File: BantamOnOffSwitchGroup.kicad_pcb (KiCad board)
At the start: 2 copper layers, 14.6 x 34 mm, 4 parts, among them J1 Conn_01x02_Male, J2 Conn_01x04_Male, SW1 SW_Push_DPDT

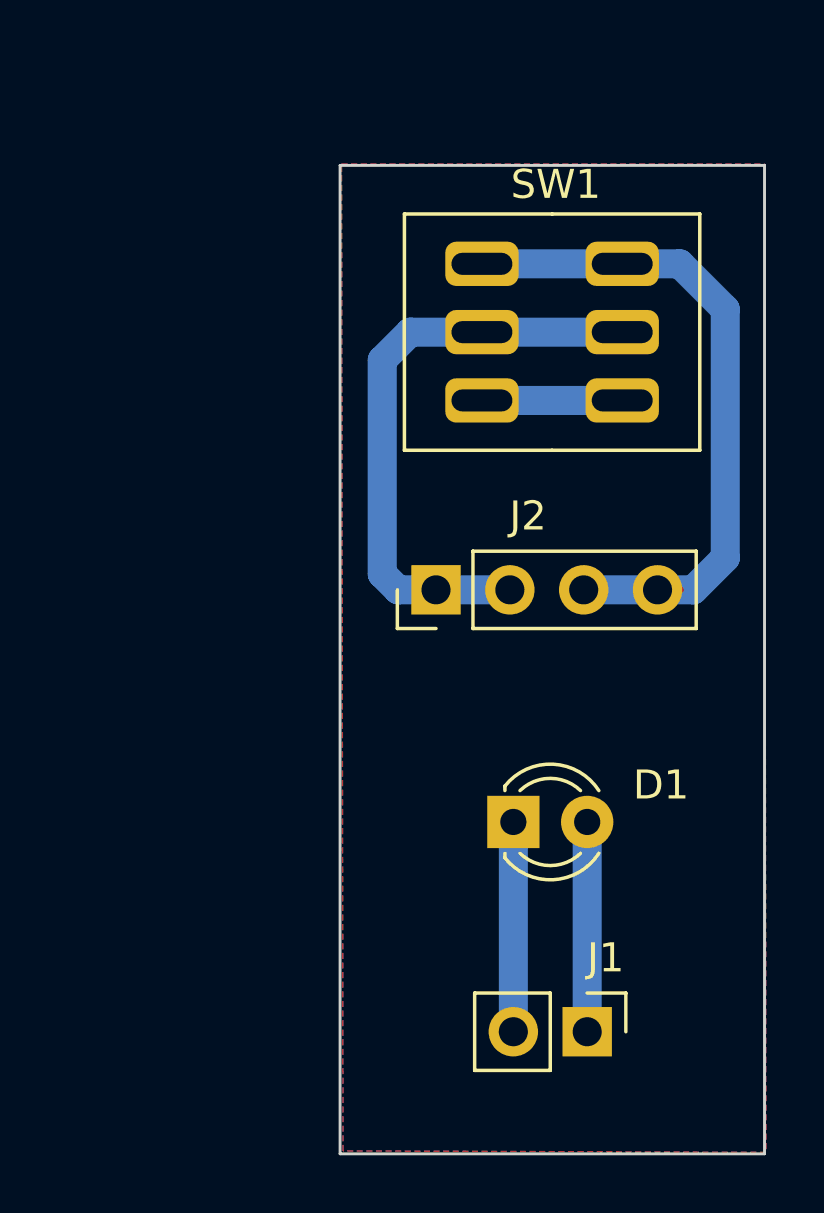
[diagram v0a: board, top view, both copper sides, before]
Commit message: gbr and drill files created
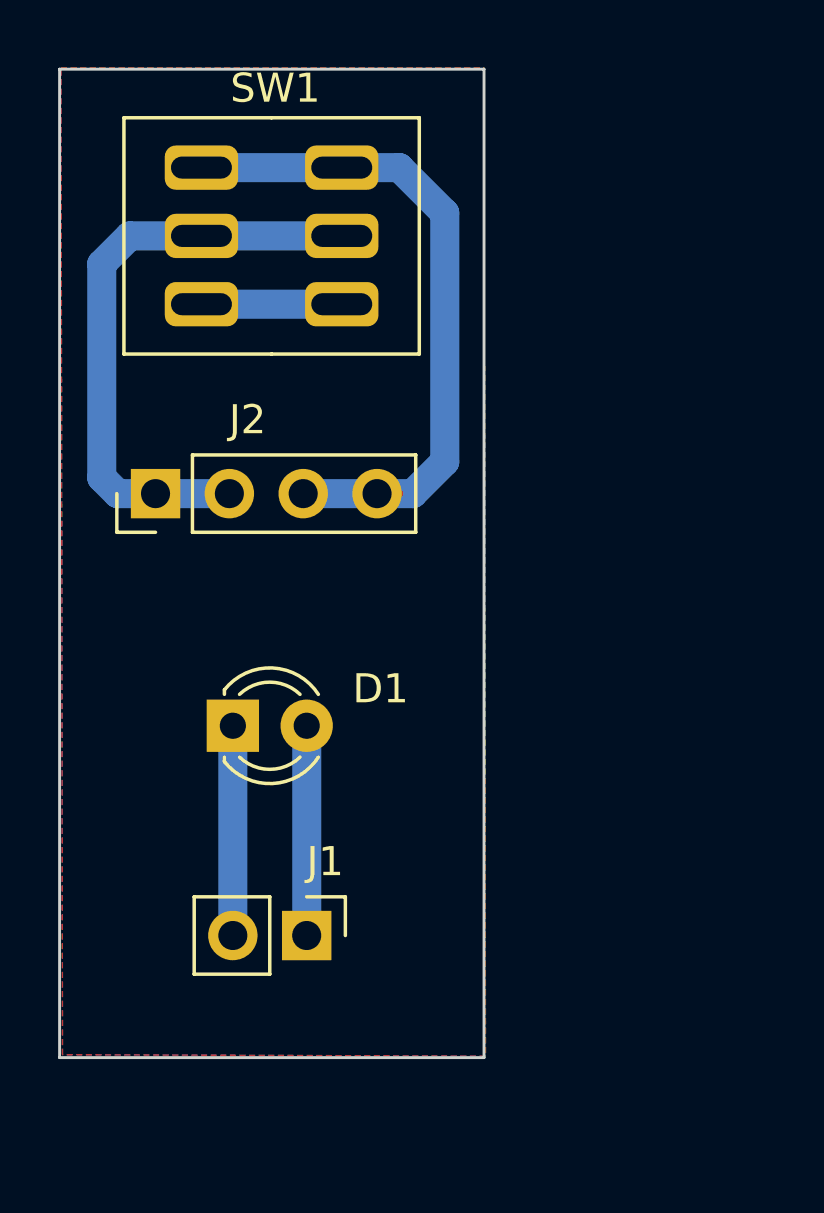
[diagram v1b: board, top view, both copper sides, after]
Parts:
- moved D1 10.2 mm to (136.2, 103.1)
- moved J1 10.2 mm to (138.8, 110.3)
- moved SW1 10.2 mm to (137.5, 86.2)
- moved J2 10.2 mm to (133.6, 95.1)
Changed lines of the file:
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@@
 		(legacy_teardrops no)
 	)
-	(paper "A4")
+	(paper "A")
+	(title_block
+		(title "Bantamp Power Switch Group")
+		(date "2024-03-06")
+		(company "RoboWidgets")
+	)
 	(layers
 		(0 "F.Cu" signal)
@@
 			(outputformat 1)
 			(mirror no)
-			(drillshape 1)
+			(drillshape 0)
 			(scaleselection 1)
-			(outputdirectory "")
+			(outputdirectory "ouput/")
 		)
 	)
@@
 	(footprint "Connector_PinHeader_2.54mm:PinHeader_1x04_P2.54mm_Vertical"
 		(layer "F.Cu")
-		(at 143.2 98.4 90)
+		(at 133.551824 95.090218 90)
 		(descr "Through hole straight pin header, 1x04, 2.54mm pitch, single row")
 		(tags "Through hole pin header THT 1x04 2.54mm single row")
@@
 	(footprint "LED_THT:LED_D3.0mm"
 		(layer "F.Cu")
-		(at 145.86 106.3845)
+		(at 136.211824 103.074718)
 		(descr "LED, diameter 3.0mm, 2 pins")
 		(tags "LED diameter 3.0mm 2 pins")
@@
 	(footprint "Connector_PinHeader_2.54mm:PinHeader_1x02_P2.54mm_Vertical"
 		(layer "F.Cu")
-		(at 148.4 113.6 -90)
+		(at 138.751824 110.290218 -90)
 		(descr "Through hole straight pin header, 1x02, 2.54mm pitch, single row")
 		(tags "Through hole pin header THT 1x02 2.54mm single row")
@@
 	(footprint "Kidwidgets:Toggle_DPDT"
 		(layer "F.Cu")
-		(at 147.193 89.535)
+		(at 137.544824 86.225218)
 		(property "Reference" "SW1"
 			(at 0.127 -5.08 0)
@@
 	)
 	(gr_rect
-		(start 139.9 83.8)
-		(end 154.5 117.8)
+		(start 130.251824 80.490218)
+		(end 144.851824 114.490218)
 		(stroke
 			(width 0.1)
@@
 	)
 	(segment
-		(start 145.86 106.3845)
-		(end 145.86 113.6)
+		(start 136.211824 103.074718)
+		(end 136.211824 110.290218)
 		(width 1)
 		(layer "B.Cu")
@@
 	)
 	(segment
-		(start 148.4 106.3845)
-		(end 148.4 113.6)
+		(start 138.751824 103.074718)
+		(end 138.751824 110.290218)
 		(width 1)
 		(layer "B.Cu")
@@
 	)
 	(segment
-		(start 143.2 98.4)
-		(end 145.74 98.4)
+		(start 133.551824 95.090218)
+		(end 136.091824 95.090218)
 		(width 1)
 		(layer "B.Cu")
@@
 	)
 	(segment
-		(start 144.78 89.535)
-		(end 142.315 89.535)
+		(start 135.131824 86.225218)
+		(end 132.666824 86.225218)
 		(width 1)
 		(layer "B.Cu")
@@
 	)
 	(segment
-		(start 141.35 97.85)
-		(end 141.9 98.4)
+		(start 131.701824 94.540218)
+		(end 132.251824 95.090218)
 		(width 1)
 		(layer "B.Cu")
@@
 	)
 	(segment
-		(start 142.315 89.535)
-		(end 141.35 90.5)
+		(start 132.666824 86.225218)
+		(end 131.701824 87.190218)
 		(width 1)
 		(layer "B.Cu")
@@
 	)
 	(segment
-		(start 149.606 89.535)
-		(end 144.78 89.535)
+		(start 139.957824 86.225218)
+		(end 135.131824 86.225218)
 		(width 1)
 		(layer "B.Cu")
@@
 	)
 	(segment
-		(start 141.35 90.5)
-		(end 141.35 97.85)
+		(start 131.701824 87.190218)
+		(end 131.701824 94.540218)
 		(width 1)
 		(layer "B.Cu")
@@
 	)
 	(segment
-		(start 141.9 98.4)
-		(end 143.2 98.4)
+		(start 132.251824 95.090218)
+		(end 133.551824 95.090218)
 		(width 1)
 		(layer "B.Cu")
@@
 	)
 	(segment
-		(start 151.6 98.4)
-		(end 150.82 98.4)
+		(start 141.951824 95.090218)
+		(end 141.171824 95.090218)
 		(width 0.25)
 		(layer "F.Cu")
@@
 	)
 	(segment
-		(start 151.5855 87.1855)
-		(end 153.15 88.75)
+		(start 141.937324 83.875718)
+		(end 143.501824 85.440218)
 		(width 1)
 		(layer "B.Cu")
@@
 	)
 	(segment
-		(start 153.15 88.75)
-		(end 153.15 97.3)
+		(start 143.501824 85.440218)
+		(end 143.501824 93.990218)
 		(width 1)
 		(layer "B.Cu")
@@
 	)
 	(segment
-		(start 153.15 97.3)
-		(end 152.05 98.4)
+		(start 143.501824 93.990218)
+		(end 142.401824 95.090218)
 		(width 1)
 		(layer "B.Cu")
@@
 	)
 	(segment
-		(start 152.05 98.4)
-		(end 150.82 98.4)
+		(start 142.401824 95.090218)
+		(end 141.171824 95.090218)
 		(width 1)
 		(layer "B.Cu")
@@
 	)
 	(segment
-		(start 144.78 87.1855)
-		(end 149.606 87.1855)
+		(start 135.131824 83.875718)
+		(end 139.957824 83.875718)
 		(width 1)
 		(layer "B.Cu")
@@
 	)
 	(segment
-		(start 148.28 98.4)
-		(end 150.82 98.4)
+		(start 138.631824 95.090218)
+		(end 141.171824 95.090218)
 		(width 1)
 		(layer "B.Cu")
@@
 	)
 	(segment
-		(start 149.606 87.1855)
-		(end 151.5855 87.1855)
+		(start 139.957824 83.875718)
+		(end 141.937324 83.875718)
 		(width 1)
 		(layer "B.Cu")
@@
 	)
 	(segment
-		(start 144.78 91.8845)
-		(end 149.606 91.8845)
+		(start 135.131824 88.574718)
+		(end 139.957824 88.574718)
 		(width 1)
 		(layer "B.Cu")
@@
 		(polygon
 			(pts
-				(xy 139.95 83.75) (xy 154.5 83.75) (xy 154.55 117.75) (xy 140 117.7)
-			)
-		)
+				(xy 130.301824 80.440218) (xy 144.851824 80.440218) (xy 144.901824 114.440218) (xy 130.351824 114.390218)
+			)
+		)
